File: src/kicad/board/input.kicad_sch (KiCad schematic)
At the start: 19 parts, among them SW1 SW_Keyboard, SW2 SW_Keyboard, SW3 RotEncoder_S, SW4 SW_Keyboard, SW5 SW_Keyboard, U2 74HC4051, U3 4072

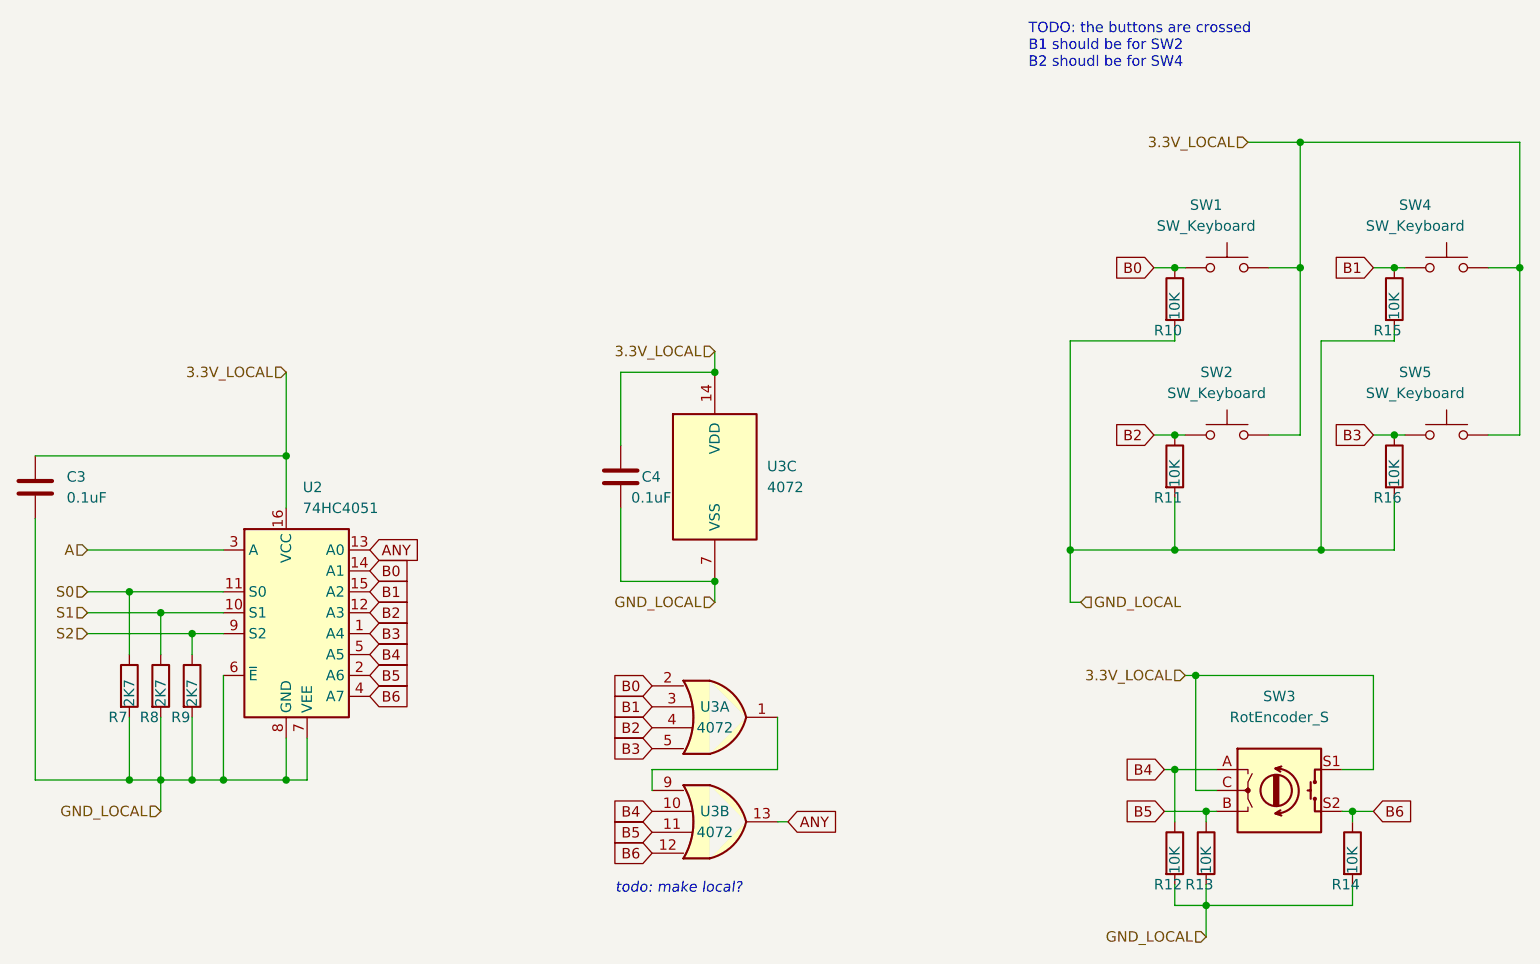
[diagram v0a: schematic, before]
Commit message: update
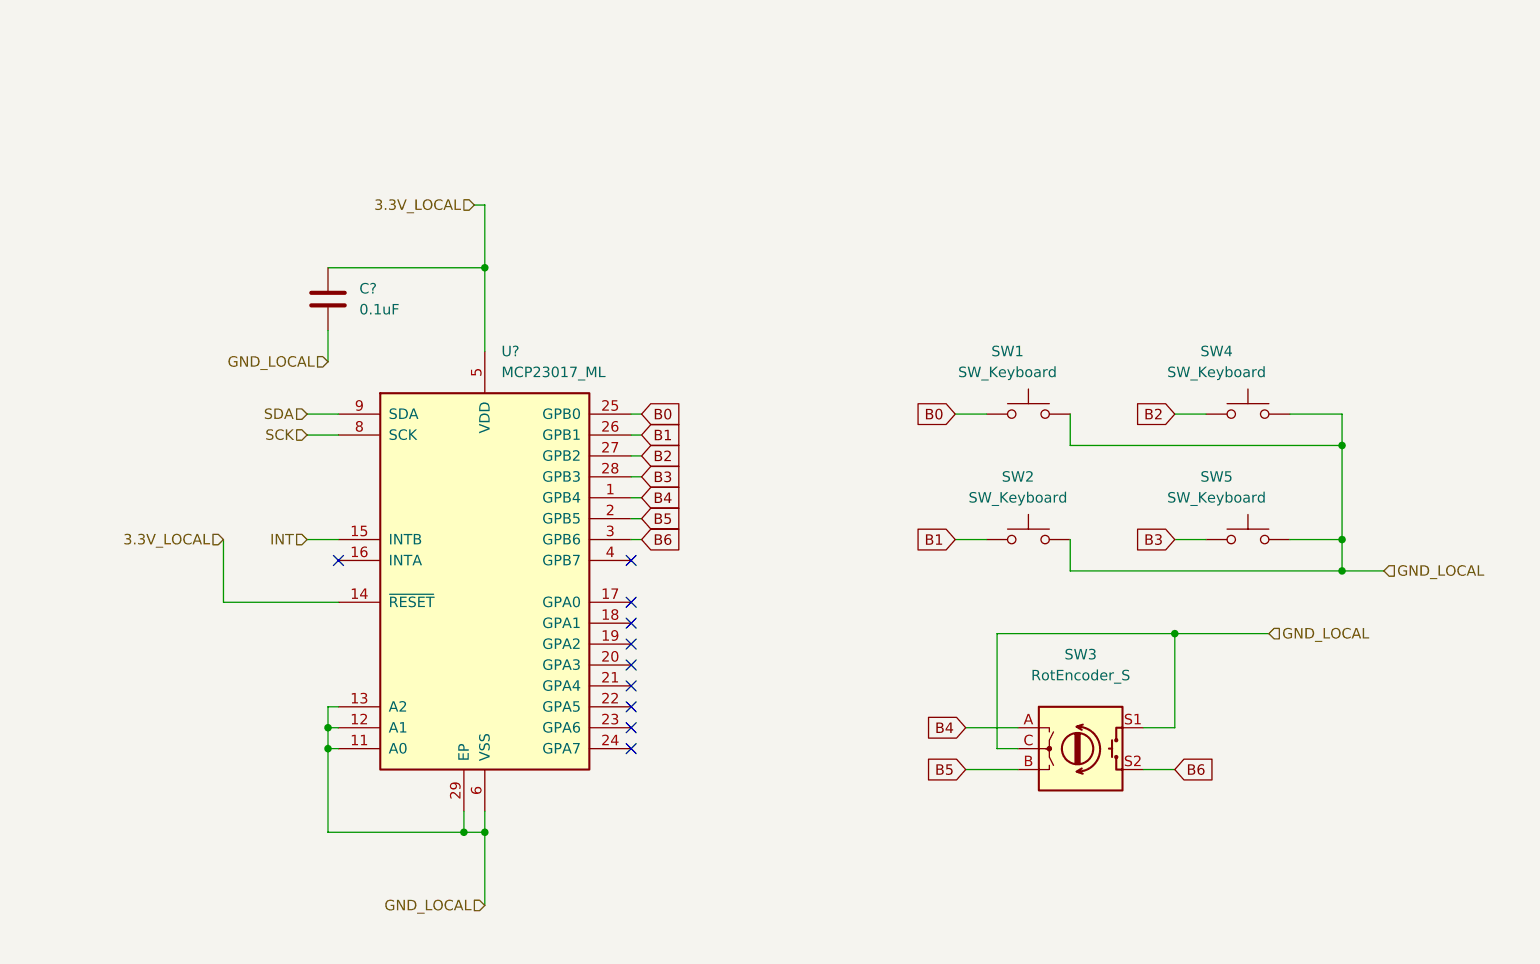
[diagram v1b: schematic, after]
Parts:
- removed C3, C4: 0.1uF, Capacitor_SMD:C_0805_2012Metric, symbol Device:C
- removed R10, R11, R12, R13, R14, R15, R16: 10K, Resistor_SMD:R_0805_2012Metric, symbol Device:R
- removed R7, R8, R9: 2K7, Resistor_SMD:R_0805_2012Metric, symbol Device:R
- removed U2: 74HC4051, Package_SO:SOIC-16_3.9x9.9mm_P1.27mm, symbol 74xx:74HC4051
- removed U3: 4072, Package_SO:SOIC-14_3.9x8.7mm_P1.27mm, symbol 4xxx:4072
- added C?: 0.1uF, Capacitor_SMD:C_0805_2012Metric, symbol Device:C
- added U?: MCP23017_ML, Package_DFN_QFN:QFN-28-1EP_6x6mm_P0.65mm_EP4.25x4.25mm, symbol Interface_Expansion:MCP23017_ML
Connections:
- net 3.3V_LOCAL: now also C?.1, U?.14 (~{RESET}), U?.5 (VDD); no longer SW1.2, SW2.2, SW3.C, SW3.S1, SW4.2, SW5.2
- net B0: now also U?.25 (GPB0)
- net B1: now also SW2.1, U?.26 (GPB1); no longer SW4.1
- net B2: now also SW4.1, U?.27 (GPB2); no longer SW2.1
- net B3: now also U?.28 (GPB3)
- net B4: now also U?.1 (GPB4)
- net B5: now also U?.2 (GPB5)
- net B6: now also U?.3 (GPB6)
- net GND_LOCAL: now also SW1.2, SW2.2, SW3.C, SW3.S1, SW4.2, SW5.2, C?.2, U?.11 (A0), U?.12 (A1), U?.13 (A2), U?.29 (EP), U?.6 (VSS)
- new net INT: U?.15 (INTB)
- new net SCK: U?.8 (SCK)
- new net SDA: U?.9 (SDA)
- no-connect marks 0 -> 10
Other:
- note removed: "TODO: the buttons are crossed B1 should be for SW2 B2 shoudl be for SW4"
- note removed: "todo: make local?"
- moved on the sheet: SW1, SW2, SW3, SW4, SW5

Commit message: update
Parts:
- U?: Vendor (none) -> C629439
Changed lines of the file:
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@@
       (effects (font (size 1.27 1.27)) (justify left) hide)
+    )
+    (property "Vendor" "C629439" (id 4) (at 118.11 96.52 0)
+      (effects (font (size 1.27 1.27)) hide)
     )
     (pin "1")
